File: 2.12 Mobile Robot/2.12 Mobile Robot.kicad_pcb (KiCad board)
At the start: 2 copper layers, 78 parts, among them J1 Motor Control R, J2 Motor Control L, J3 GND, J4 Motor Power R, J5 Battery Power, J6 Motor Power L, J7 3.3V, J8 UART, J9 5V, Q1 DMMT5401-7-F, Q2 DMG2305UX-13, SW1 SW_PWR, SW2 RST_SW, SW3 BOOT_SW, SW4 SW_PWR, U1 MOTOR_PWR, U2 ProS3, U3 TCA9548APWR, U4 POWER_IN, U5 TPS564208DDCT

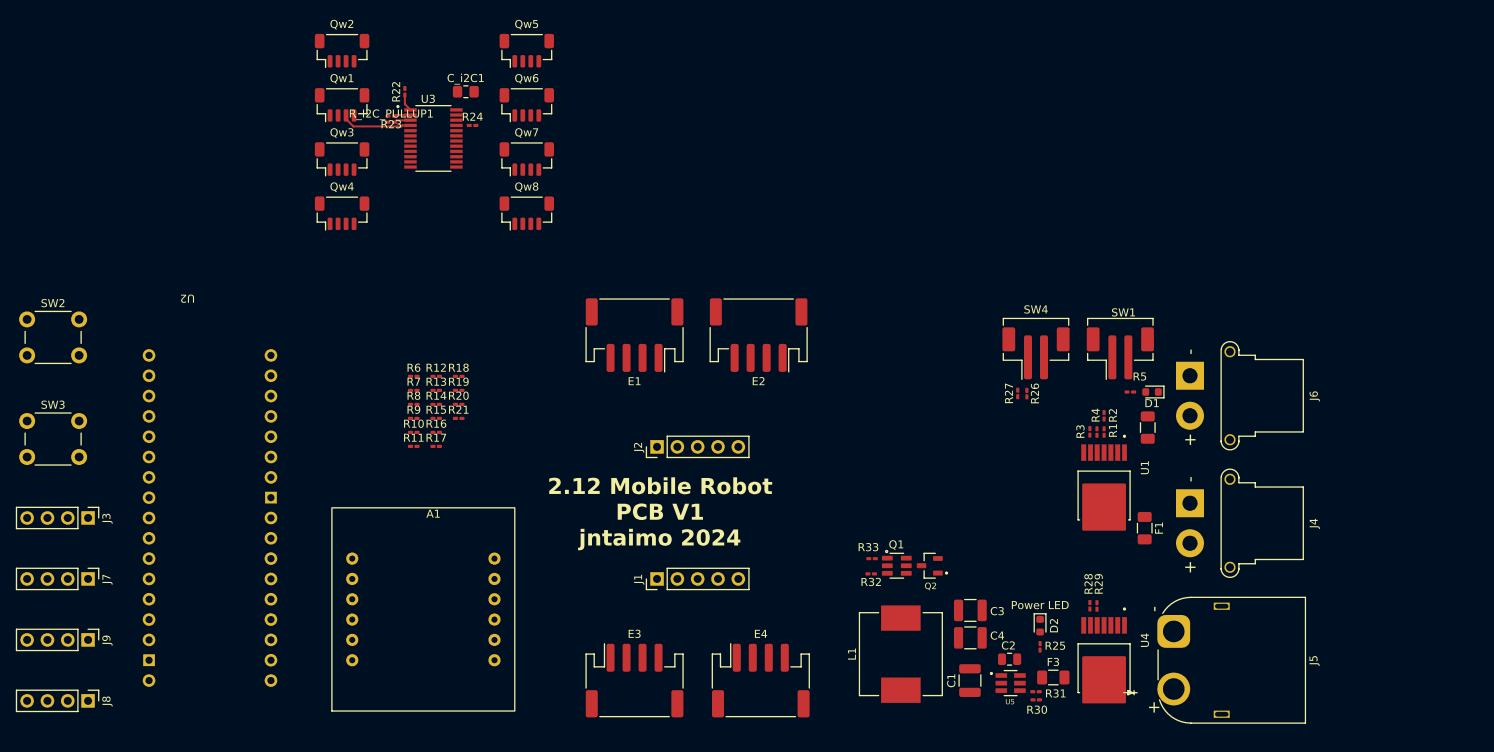
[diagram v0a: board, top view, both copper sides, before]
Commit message: Fully routed
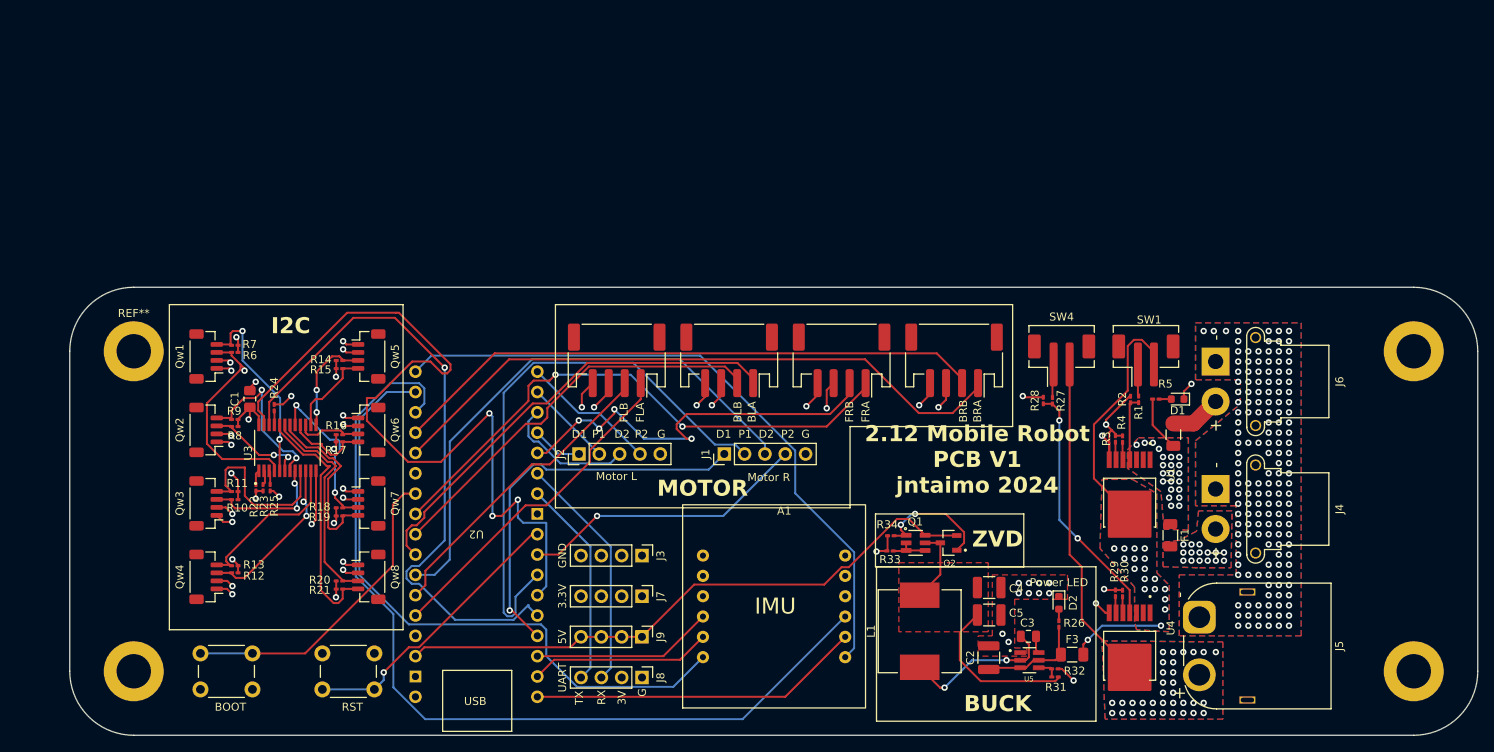
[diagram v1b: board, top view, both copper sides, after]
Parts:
- added ?: , , F.Cu at (200.0, 136.0)
- added ?: , , F.Cu at (40.0, 136.0)
- added ?: , , F.Cu at (200.0, 96.0)
- added REF**: MountingHole_4.3mm_M4_DIN965_Pad, MountingHole:MountingHole_4.3mm_M4_DIN965_Pad, F.Cu at (40.0, 96.0)
- J1: value Motor Control R -> Motor R
- J2: value Motor Control L -> Motor L
- SW2: value RST_SW -> RST
- SW3: value BOOT_SW -> BOOT
- moved J3 69.4 mm to (103.5, 121.5)
- moved J8 69.3 mm to (103.5, 136.8)
- moved J7 69.3 mm to (103.5, 126.6)
- moved J9 69.2 mm to (103.5, 131.7)
- moved SW2 55.7 mm to (63.6, 133.8)
- moved R22 52.9 mm to (55.3, 113.1), turned to -90 degrees
- moved Qw2 50.4 mm to (49.0, 105.8), turned to 90 degrees
- moved Qw8 49.6 mm to (69.4, 124.2), turned to -90 degrees
- moved R23 49.1 mm to (56.2, 113.1), turned to -90 degrees
- moved Qw4 48.5 mm to (49.0, 124.2), turned to 90 degrees
- moved R25 48.1 mm to (57.0, 113.1), turned to 90 degrees
- moved E3 47.7 mm to (128.5, 97.1), turned to 180 degrees
- moved Qw7 47.4 mm to (69.4, 115.0), turned to -90 degrees
- moved C1 46.9 mm to (54.5, 102.0), turned to 90 degrees
- moved E4 46.7 mm to (142.5, 97.1), turned to 180 degrees
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- renumbered C_i2C1 to C1, C1 to C2, C2 to C3, C3 to C4, C4 to C5, R_I2C_PULLUP1 to R25, R25 to R26, R26 to R27, R27 to R28, R28 to R29, R29 to R30, R30 to R31, R31 to R32, R32 to R33, R33 to R34
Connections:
- net Net-(F1-Pad2) renamed /R_MOTOR
- net Net-(F2-Pad2) renamed /L_MOTOR
- F3 pad 1: /Buck/VBAT -> /VBAT
- U4 pad 1: /Buck/VBAT -> /VBAT
- U4 pad 2: /Buck/VBAT -> /VBAT
- U4 pad 3: /Buck/VBAT -> /VBAT
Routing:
- net /IMU_RST: track 0.00 -> 113.2 mm
- net /SDA: track 0.00 -> 103.7 mm, vias 0 -> 3
- net /IMU_CS: track 0.00 -> 82.6 mm
- net /SCL: track 0.00 -> 80.5 mm, vias 0 -> 1
- net /IMU_INT: track 0.00 -> 80.1 mm
- net /HALL_BR_A: track 0.00 -> 79.8 mm
- net +5V: track 0.00 -> 75.6 mm
- net /HALL_BR_B: track 0.00 -> 74.3 mm
- net GND: track 0.00 -> 72.9 mm, vias 0 -> 189
- net /PWM1_R: track 0.00 -> 71.6 mm
- net /HALL_FR_A: track 0.00 -> 69.8 mm, vias 0 -> 2
- net /DIR2_R: track 0.00 -> 69.1 mm
- net /HALL_BL_A: track 0.00 -> 57.3 mm
- net +3.3V: track 0.00 -> 54.5 mm, vias 0 -> 21
- net /HALL_FR_B: track 0.00 -> 51.8 mm, vias 0 -> 4
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- added copper zone on In2.Cu, net +3.3V
- added copper zone on F.Cu, net /BUCK_5V
- added copper zone on In1.Cu, net /BUCK_5V
- added copper zone on In2.Cu, net /BUCK_5V
- added copper zone on B.Cu, net /R_MOTOR
- added copper zone on F.Cu, net /R_MOTOR
- added copper zone on In1.Cu, net /R_MOTOR
- added copper zone on In2.Cu, net /R_MOTOR
- added copper zone on B.Cu, net /VBAT
- added copper zone on F.Cu, net /VBAT
- added copper zone on In1.Cu, net /VBAT
- added copper zone on In2.Cu, net /VBAT
- added copper zone on B.Cu, net /VBAT_IN
- added copper zone on F.Cu, net /VBAT_IN
- added copper zone on In1.Cu, net /VBAT_IN
- added copper zone on In2.Cu, net /VBAT_IN
- added copper zone on B.Cu, net /VBAT_MOTOR
- added copper zone on F.Cu, net /VBAT_MOTOR
- added copper zone on In1.Cu, net /VBAT_MOTOR
- added copper zone on In2.Cu, net /VBAT_MOTOR
- added copper zone on B.Cu, net GND
- added copper zone on F.Cu, net GND
- added copper zone on In1.Cu, net GND
- added copper zone on In2.Cu, net GND
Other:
- board outline added: 176 x 56 mm
- copper layers 2 -> 4
- board text added: "3V"
- board text added: "BLA"
- board text added: "BLB"
- board text added: "BRA"
- board text added: "BRB"
- board text added: "BUCK"
- board text added: "D1"
- board text added: "D2"
- board text added: "FLA"
- board text added: "FLB"
- board text added: "FRA"
- board text added: "FRB"
- board text added: "G"
- board text added: "I2C"
- board text added: "IMU"
- board text added: "MOTOR"
- board text added: "P1"
- board text added: "P2"
- board text added: "RX"
- board text added: "TX"
- board text added: "USB"
- board text added: "ZVD"
